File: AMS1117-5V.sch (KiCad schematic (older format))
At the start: 7 parts, among them J6 Conn_01x03, U3 AMS1117-5.0

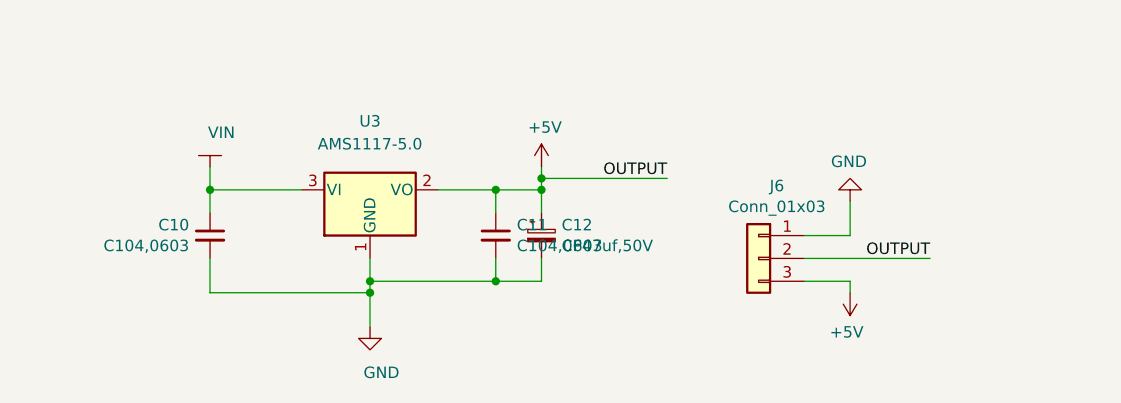
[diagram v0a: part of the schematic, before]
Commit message: update,
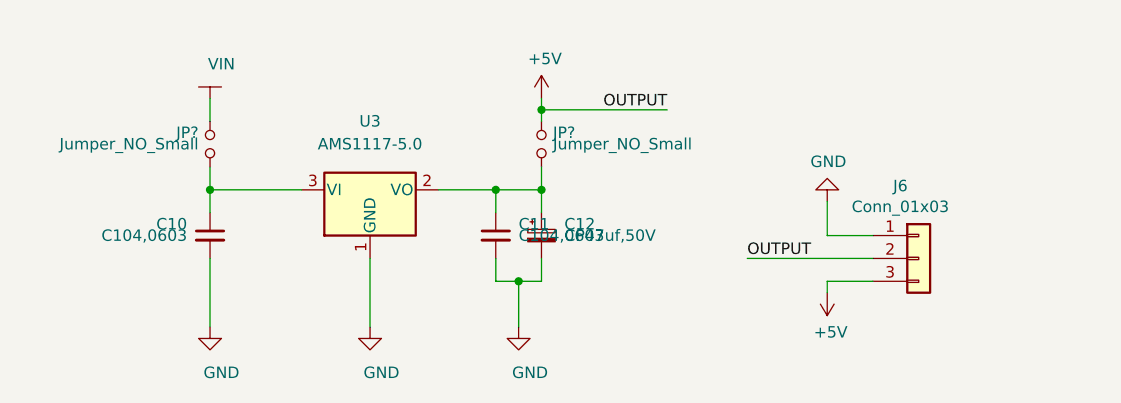
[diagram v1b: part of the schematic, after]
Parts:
- added JP? (x2): Jumper_NO_Small, symbol Device:Jumper_NO_Small
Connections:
- net +5V: now also JP?.1; no longer C11.1, C12.1, U3.2 (VO)
- net VIN: now also JP?.1; no longer C10.1, U3.3 (VI)
- new net: C11.1, C12.1, JP?.2, U3.2 (VO)
- new net: C10.1, JP?.2, U3.3 (VI)
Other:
- moved on the sheet: J6
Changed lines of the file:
@@
 AR Path="/5C0BBB2B/5C0D4462" Ref="C?"  Part="1"
 AR Path="/5C0BFA48/5C0D4462" Ref="C10"  Part="1"
-F 0 "C10" H 1259 1596 50  0000 R CNN
-F 1 "C104,0603" H 1259 1505 50  0000 R CNN
+F 0 "C10" H 1250 1600 50  0000 R CNN
+F 1 "C104,0603" H 1250 1550 50  0000 R CNN
 F 2 "Capacitor_SMD:C_0603_1608Metric_Pad1.05x0.95mm_HandSolder" H 1350 1550 50  0001 C CNN
 F 3 "~" H 1350 1550 50  0001 C CNN
@@
 $EndComp
 Wire Wire Line
-	1350 1650 1350 1800
-Wire Wire Line
-	1350 1800 2050 1800
-Wire Wire Line
-	2050 1800 2050 1950
-Wire Wire Line
-	2050 1650 2050 1750
-Connection ~ 2050 1800
-Wire Wire Line
-	2050 1750 2600 1750
-Wire Wire Line
 	2800 1750 2800 1650
-Connection ~ 2050 1750
-Wire Wire Line
-	2050 1750 2050 1800
 $Comp
 L power:+5V #PWR?
 U 1 1 5C0AD768
-P 2800 1250
+P 2800 950
 AR Path="/5C0BBB2B/5C0AD768" Ref="#PWR?"  Part="1"
 AR Path="/5C0BFA48/5C0AD768" Ref="#PWR0122"  Part="1"
-F 0 "#PWR0122" H 2800 1100 50  0001 C CNN
-F 1 "+5V" H 2815 1423 50  0000 C CNN
-F 2 "" H 2800 1250 50  0001 C CNN
-F 3 "" H 2800 1250 50  0001 C CNN
-	1    2800 1250
+F 0 "#PWR0122" H 2800 800 50  0001 C CNN
+F 1 "+5V" H 2815 1123 50  0000 C CNN
+F 2 "" H 2800 950 50  0001 C CNN
+F 3 "" H 2800 950 50  0001 C CNN
+	1    2800 950
 	1    0    0    -1
 $EndComp
@@
 Wire Wire Line
 	1350 1350 1350 1450
-Wire Wire Line
-	2800 1250 2800 1300
 Wire Wire Line
 	2350 1350 2600 1350
@@
 AR Path="/5C0BBB2B/5C0AD77C" Ref="C?"  Part="1"
 AR Path="/5C0BFA48/5C0AD77C" Ref="C11"  Part="1"
-F 0 "C11" H 2692 1596 50  0000 L CNN
-F 1 "C104,0603" H 2692 1505 50  0000 L CNN
+F 0 "C11" H 2700 1600 50  0000 L CNN
+F 1 "C104,0603" H 2700 1550 50  0000 L CNN
 F 2 "Capacitor_SMD:C_0603_1608Metric_Pad1.05x0.95mm_HandSolder" H 2600 1550 50  0001 C CNN
 F 3 "~" H 2600 1550 50  0001 C CNN
@@
 Wire Wire Line
 	2600 1650 2600 1750
-Connection ~ 2600 1750
-Wire Wire Line
-	2600 1750 2800 1750
+Wire Wire Line
+	2600 1750 2700 1750
 $Comp
 L taobao-cp:CP47uf,50V C?
@@
 AR Path="/5C0BBB2B/5C0D445F" Ref="C?"  Part="1"
 AR Path="/5C0BFA48/5C0D445F" Ref="C12"  Part="1"
-F 0 "C12" H 2888 1596 50  0000 L CNN
-F 1 "CP47uf,50V" H 2888 1505 50  0000 L CNN
+F 0 "C12" H 2900 1600 50  0000 L CNN
+F 1 "CP47uf,50V" H 2900 1550 50  0000 L CNN
 F 2 "w_smd_cap:c_elec_6.3x7.7" H 2800 1550 50  0001 C CNN
 F 3 "~" H 2800 1550 50  0001 C CNN
@@
 L Connector_Generic:Conn_01x03 J?
 U 1 1 5C0D4460
-P 3750 1650
+P 4450 1650
 AR Path="/5C0BBB2B/5C0D4460" Ref="J?"  Part="1"
 AR Path="/5C0BFA48/5C0D4460" Ref="J6"  Part="1"
-F 0 "J6" H 3670 1967 50  0000 C CNN
-F 1 "Conn_01x03" H 3670 1876 50  0000 C CNN
-F 2 "Connector_PinHeader_2.54mm:PinHeader_1x03_P2.54mm_Vertical" H 3750 1650 50  0001 C CNN
-F 3 "~" H 3750 1650 50  0001 C CNN
-	1    3750 1650
-	-1   0    0    -1
+F 0 "J6" H 4370 1967 50  0000 C CNN
+F 1 "Conn_01x03" H 4370 1876 50  0000 C CNN
+F 2 "Connector_PinHeader_2.54mm:PinHeader_1x03_P2.54mm_Vertical" H 4450 1650 50  0001 C CNN
+F 3 "~" H 4450 1650 50  0001 C CNN
+	1    4450 1650
+	1    0    0    -1
 $EndComp
 $Comp
 L power:GND #PWR?
 U 1 1 5C0D4461
-P 4150 1400
+P 4050 1400
 AR Path="/5C0BBB2B/5C0D4461" Ref="#PWR?"  Part="1"
 AR Path="/5C0BFA48/5C0D4461" Ref="#PWR0123"  Part="1"
-F 0 "#PWR0123" H 4150 1150 50  0001 C CNN
-F 1 "GND" H 4155 1227 50  0000 C CNN
-F 2 "" H 4150 1400 50  0001 C CNN
-F 3 "" H 4150 1400 50  0001 C CNN
-	1    4150 1400
-	-1   0    0    1
-$EndComp
-Wire Wire Line
-	3950 1550 4150 1550
-Wire Wire Line
-	4150 1550 4150 1400
+F 0 "#PWR0123" H 4050 1150 50  0001 C CNN
+F 1 "GND" H 4055 1227 50  0000 C CNN
+F 2 "" H 4050 1400 50  0001 C CNN
+F 3 "" H 4050 1400 50  0001 C CNN
+	1    4050 1400
+	1    0    0    1
+$EndComp
+Wire Wire Line
+	4250 1550 4050 1550
+Wire Wire Line
+	4050 1550 4050 1400
 $Comp
 L power:+5V #PWR?
 U 1 1 5C078B67
-P 4150 1800
+P 4050 1800
 AR Path="/5C0BBB2B/5C078B67" Ref="#PWR?"  Part="1"
 AR Path="/5C0BFA48/5C078B67" Ref="#PWR0124"  Part="1"
-F 0 "#PWR0124" H 4150 1650 50  0001 C CNN
-F 1 "+5V" H 4165 1973 50  0000 C CNN
-F 2 "" H 4150 1800 50  0001 C CNN
-F 3 "" H 4150 1800 50  0001 C CNN
-	1    4150 1800
-	-1   0    0    1
-$EndComp
-Wire Wire Line
-	3950 1750 4150 1750
-Wire Wire Line
-	4150 1750 4150 1800
-Text Label 3350 1300 2    50   ~ 0
+F 0 "#PWR0124" H 4050 1650 50  0001 C CNN
+F 1 "+5V" H 4065 1973 50  0000 C CNN
+F 2 "" H 4050 1800 50  0001 C CNN
+F 3 "" H 4050 1800 50  0001 C CNN
+	1    4050 1800
+	1    0    0    1
+$EndComp
+Wire Wire Line
+	4250 1750 4050 1750
+Wire Wire Line
+	4050 1750 4050 1800
+Text Label 3350 1000 2    50   ~ 0
 OUTPUT
 Wire Wire Line
-	2800 1300 3350 1300
-Connection ~ 2800 1300
-Wire Wire Line
-	2800 1300 2800 1350
-Text Label 4500 1650 2    50   ~ 0
+	2800 1000 3350 1000
+Text Label 3700 1650 0    50   ~ 0
 OUTPUT
 Wire Wire Line
-	3950 1650 4500 1650
+	4250 1650 3700 1650
 $Comp
 L power:+5V #PWR?
@@
 L taobao-components:VIN #PWR0127
 U 1 1 5C0C05CD
-P 1350 1250
-F 0 "#PWR0127" H 1350 1100 50  0001 C CNN
-F 1 "VIN" H 1400 1400 50  0000 C CNN
-F 2 "" H 1350 1250 50  0001 C CNN
-F 3 "" H 1350 1250 50  0001 C CNN
-	1    1350 1250
+P 1350 950
+F 0 "#PWR0127" H 1350 800 50  0001 C CNN
+F 1 "VIN" H 1400 1100 50  0000 C CNN
+F 2 "" H 1350 950 50  0001 C CNN
+F 3 "" H 1350 950 50  0001 C CNN
+	1    1350 950
 	1    0    0    -1
 $EndComp
@@
 	0    -1   -1   0
 $EndComp
+$Comp
+L Device:Jumper_NO_Small JP?
+U 1 1 5C146472
+P 2800 1150
+F 0 "JP?" V 2750 1200 50  0000 L CNN
+F 1 "Jumper_NO_Small" V 2800 1200 50  0000 L CNN
+F 2 "" H 2800 1150 50  0001 C CNN
+F 3 "~" H 2800 1150 50  0001 C CNN
+	1    2800 1150
+	0    1    1    0
+$EndComp
+Wire Wire Line
+	2800 950  2800 1000
+$Comp
+L Device:Jumper_NO_Small JP?
+U 1 1 5C146BBB
+P 1350 1150
+F 0 "JP?" V 1300 1100 50  0000 R CNN
+F 1 "Jumper_NO_Small" V 1350 1100 50  0000 R CNN
+F 2 "" H 1350 1150 50  0001 C CNN
+F 3 "~" H 1350 1150 50  0001 C CNN
+	1    1350 1150
+	0    1    1    0
+$EndComp
+Wire Wire Line
+	1350 950  1350 1050
+Connection ~ 2800 1000
+Wire Wire Line
+	2800 1000 2800 1050
+Wire Wire Line
+	2800 1250 2800 1350
+Wire Wire Line
+	2050 1650 2050 1950
+$Comp
+L power:GND #PWR?
+U 1 1 5C14C4BF
+P 1350 1950
+AR Path="/5C0BBB2B/5C14C4BF" Ref="#PWR?"  Part="1"
+AR Path="/5C0BFA48/5C14C4BF" Ref="#PWR?"  Part="1"
+F 0 "#PWR?" H 1350 1700 50  0001 C CNN
+F 1 "GND" H 1400 1750 50  0000 C CNN
+F 2 "" H 1350 1950 50  0001 C CNN
+F 3 "" H 1350 1950 50  0001 C CNN
+	1    1350 1950
+	1    0    0    -1
+$EndComp
+Wire Wire Line
+	1350 1650 1350 1950
+$Comp
+L power:GND #PWR?
+U 1 1 5C14CA96
+P 2700 1950
+AR Path="/5C0BBB2B/5C14CA96" Ref="#PWR?"  Part="1"
+AR Path="/5C0BFA48/5C14CA96" Ref="#PWR?"  Part="1"
+F 0 "#PWR?" H 2700 1700 50  0001 C CNN
+F 1 "GND" H 2750 1750 50  0000 C CNN
+F 2 "" H 2700 1950 50  0001 C CNN
+F 3 "" H 2700 1950 50  0001 C CNN
+	1    2700 1950
+	1    0    0    -1
+$EndComp
+Wire Wire Line
+	2700 1950 2700 1750
+Connection ~ 2700 1750
+Wire Wire Line
+	2700 1750 2800 1750
 $EndSCHEMATC

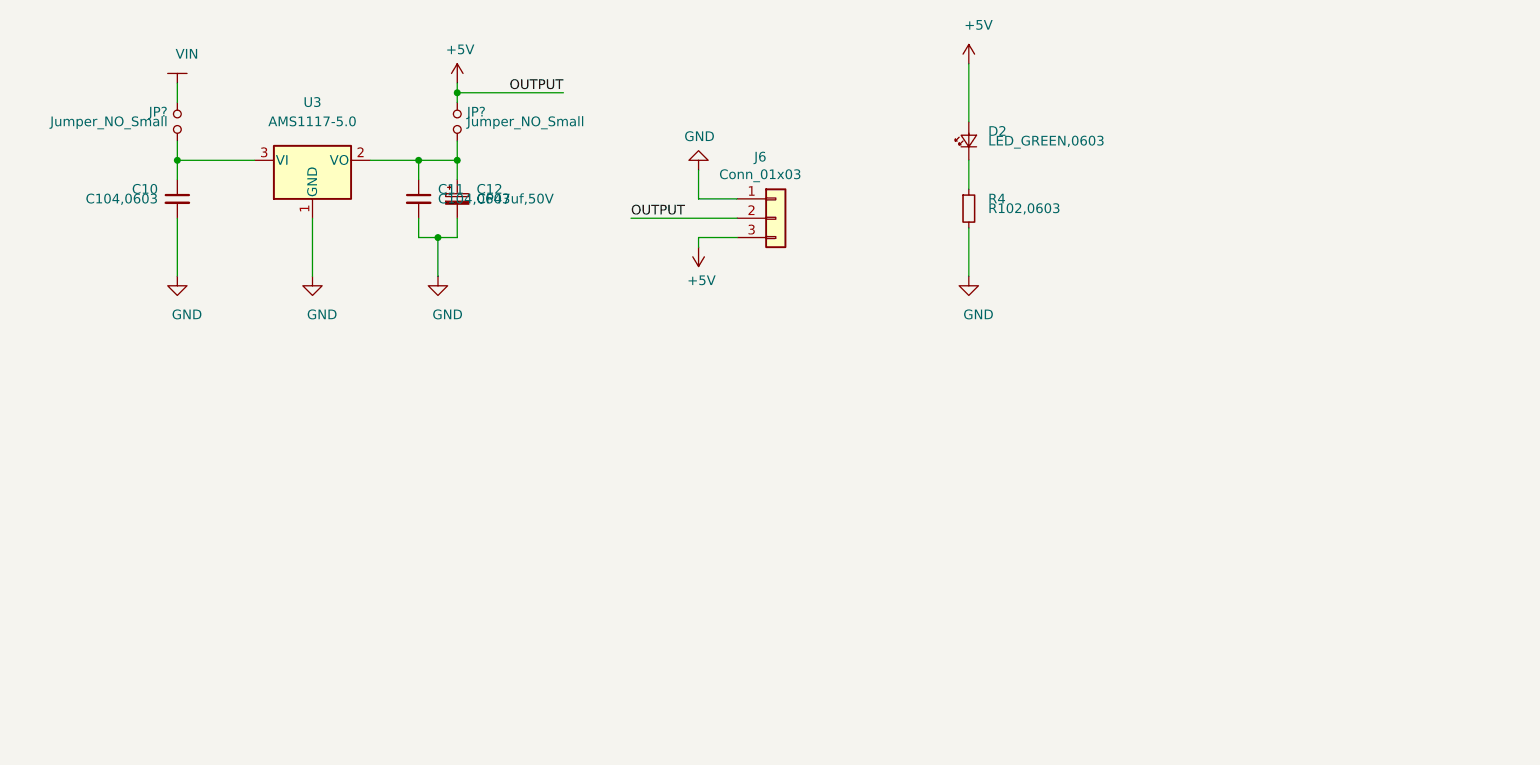
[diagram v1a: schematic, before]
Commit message: update,
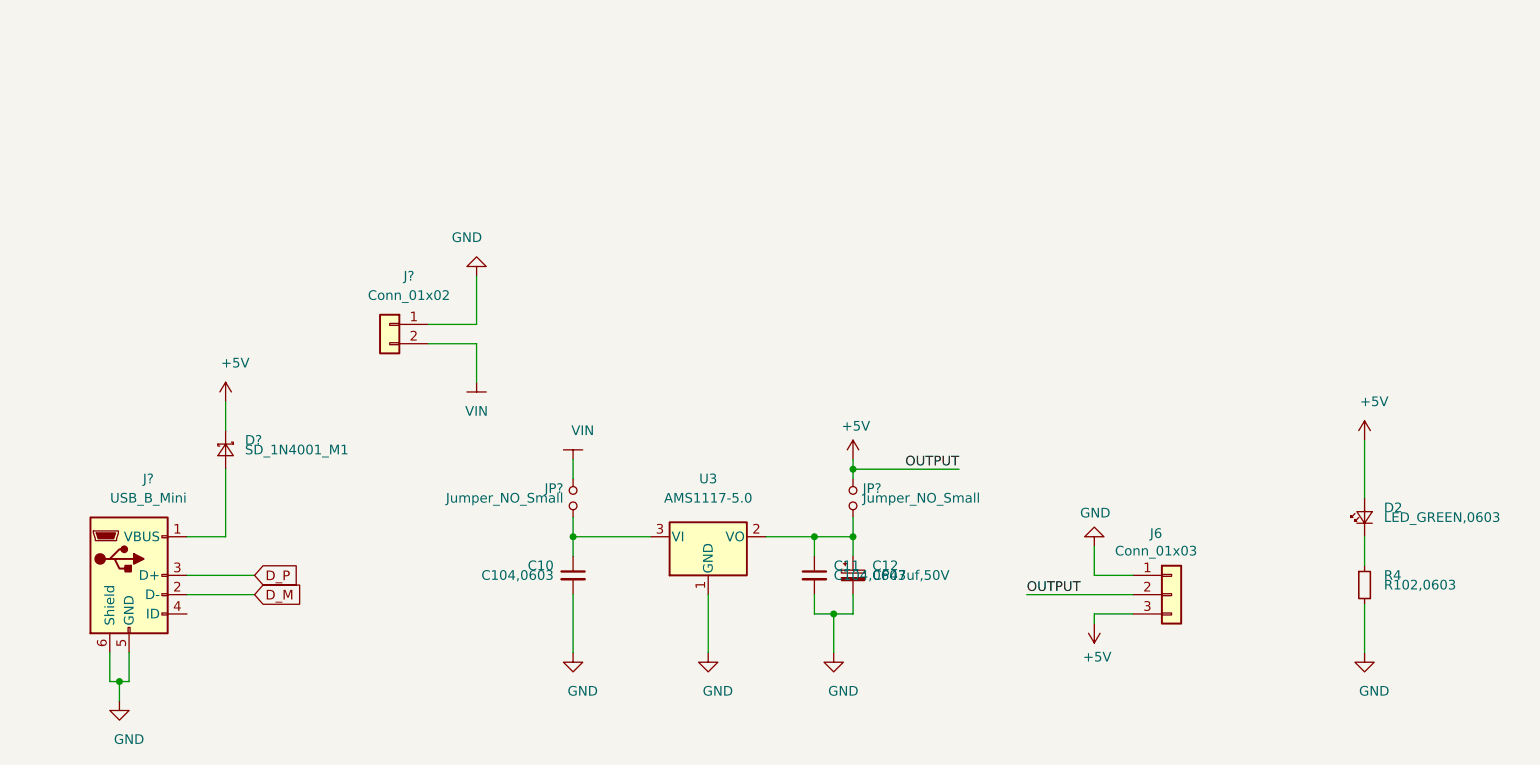
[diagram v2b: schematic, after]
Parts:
- added D?: SD_1N4001_M1, w_smd_diode:do214ac, symbol taobao-sd:SD_1N4001_M1
- added J?: USB_B_Mini, Connector_USB:USB_Micro-B_Amphenol_10103594-0001LF_Horizontal, symbol Connector:USB_B_Mini
- added J?: Conn_01x02, symbol Connector_Generic:Conn_01x02
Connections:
- net +5V: now also D?.1 (K)
- net GND: now also J?.1 (Pin_1), J?.5 (GND), J?.6 (Shield)
- net VIN: now also J?.2 (Pin_2)
- new net: D?.2 (A), J?.1 (VBUS)
- new net D_M: J?.2 (D-)
- new net D_P: J?.3 (D+)
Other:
- moved on the sheet: C10, C11, C12, D2, J6, JP?, R4, U3
